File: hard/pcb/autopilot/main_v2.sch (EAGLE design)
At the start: 168 parts, among them IC1 24AA32ASN, IC2 INA194, IC3 LP2950Z, Q1 IRLML5203, Q3 IRLML5203, Q4 IRLML5203, T3 BC848, U2 TMP75DGK, U44 BMP085, X1 USB-SMD-NS

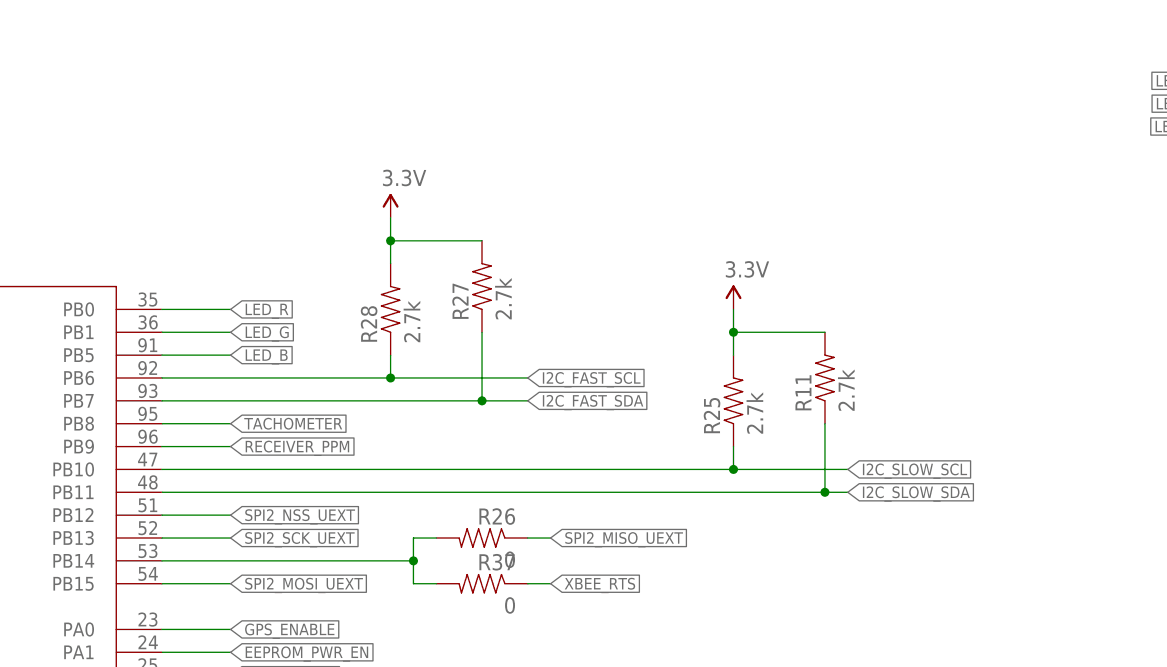
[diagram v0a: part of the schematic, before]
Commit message: nop
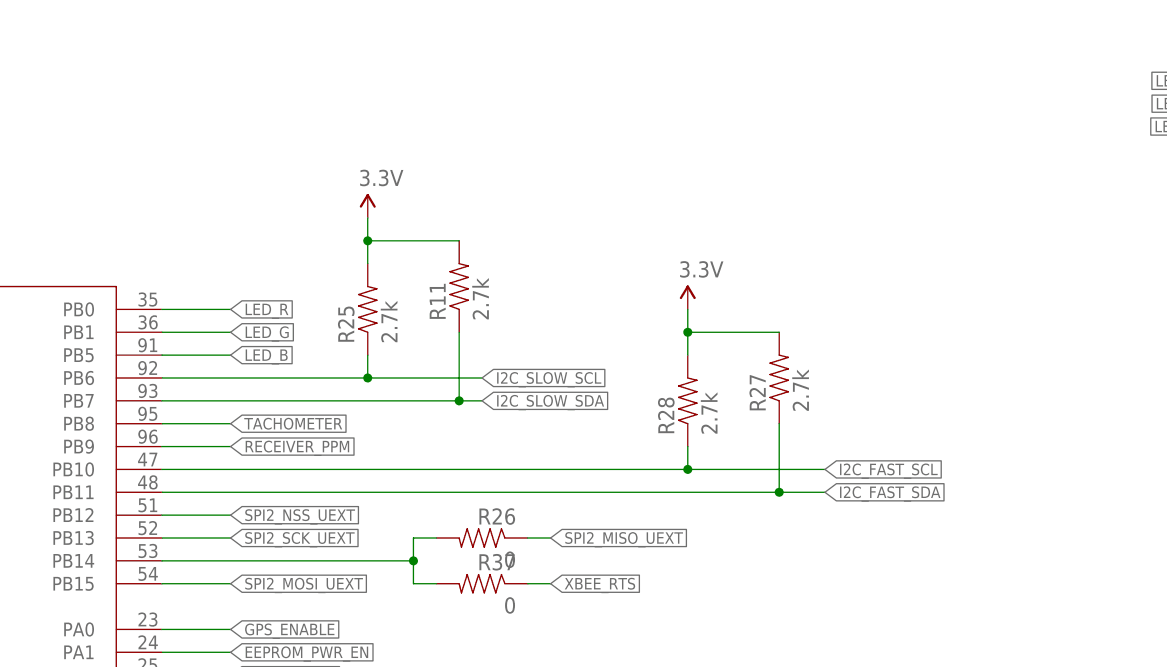
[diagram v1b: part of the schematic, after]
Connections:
- net I2C_FAST_SCL: now also DD1.PB10; no longer DD1.PB6
- net I2C_FAST_SDA: now also DD1.PB11; no longer DD1.PB7
- net I2C_SLOW_SCL: now also DD1.PB6; no longer DD1.PB10
- net I2C_SLOW_SDA: now also DD1.PB7; no longer DD1.PB11
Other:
- moved on the sheet: R11, R25, R27, R28
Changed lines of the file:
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@@
 <setting verticaltext="up"/>
 </settings>
-<grid distance="0.1" unitdist="inch" unit="inch" style="lines" multiple="1" display="no" altdistance="0.01" altunitdist="inch" altunit="inch"/>
+<grid distance="0.1" unitdist="inch" unit="inch" style="lines" multiple="1" display="yes" altdistance="0.01" altunitdist="inch" altunit="inch"/>
 <layers>
 <layer number="1" name="Top" color="4" fill="1" visible="no" active="no"/>
@@
 <instance part="P+18" gate="G$1" x="-218.44" y="2.54"/>
 <instance part="GND31" gate="1" x="-218.44" y="-20.32"/>
-<instance part="R27" gate="G$1" x="76.2" y="78.74" rot="R90"/>
-<instance part="P+16" gate="G$1" x="66.04" y="86.36"/>
-<instance part="R28" gate="G$1" x="66.04" y="76.2" rot="R90"/>
+<instance part="R27" gate="G$1" x="109.22" y="68.58" rot="R90"/>
+<instance part="P+16" gate="G$1" x="99.06" y="76.2"/>
+<instance part="R28" gate="G$1" x="99.06" y="66.04" rot="R90"/>
 <instance part="U44" gate="G$1" x="309.88" y="17.78"/>
 <instance part="U2" gate="G$1" x="309.88" y="-12.7"/>
@@
 <instance part="C37" gate="G$1" x="106.68" y="-55.88" rot="MR180"/>
 <instance part="C39" gate="G$1" x="86.36" y="-55.88" rot="MR180"/>
-<instance part="R11" gate="G$1" x="114.3" y="68.58" rot="R90"/>
-<instance part="P+20" gate="G$1" x="104.14" y="76.2"/>
-<instance part="R25" gate="G$1" x="104.14" y="66.04" rot="R90"/>
+<instance part="R11" gate="G$1" x="73.66" y="78.74" rot="R90"/>
+<instance part="P+20" gate="G$1" x="63.5" y="86.36"/>
+<instance part="R25" gate="G$1" x="63.5" y="76.2" rot="R90"/>
 <instance part="R26" gate="G$1" x="76.2" y="50.8" rot="MR0"/>
 <instance part="R37" gate="G$1" x="76.2" y="45.72" rot="MR0"/>
@@
 </segment>
 <segment>
-<wire x1="66.04" y1="86.36" x2="66.04" y2="83.82" width="0.1524" layer="91"/>
-<wire x1="66.04" y1="83.82" x2="66.04" y2="81.28" width="0.1524" layer="91"/>
-<wire x1="66.04" y1="83.82" x2="76.2" y2="83.82" width="0.1524" layer="91"/>
-<junction x="66.04" y="83.82"/>
+<wire x1="99.06" y1="76.2" x2="99.06" y2="73.66" width="0.1524" layer="91"/>
+<wire x1="99.06" y1="73.66" x2="99.06" y2="71.12" width="0.1524" layer="91"/>
+<wire x1="99.06" y1="73.66" x2="109.22" y2="73.66" width="0.1524" layer="91"/>
+<junction x="99.06" y="73.66"/>
 <pinref part="P+16" gate="G$1" pin="3.3V"/>
 <pinref part="R28" gate="G$1" pin="2"/>
@@
 </segment>
 <segment>
-<wire x1="104.14" y1="76.2" x2="104.14" y2="73.66" width="0.1524" layer="91"/>
-<wire x1="104.14" y1="73.66" x2="104.14" y2="71.12" width="0.1524" layer="91"/>
-<wire x1="104.14" y1="73.66" x2="114.3" y2="73.66" width="0.1524" layer="91"/>
-<junction x="104.14" y="73.66"/>
+<wire x1="63.5" y1="86.36" x2="63.5" y2="83.82" width="0.1524" layer="91"/>
+<wire x1="63.5" y1="83.82" x2="63.5" y2="81.28" width="0.1524" layer="91"/>
+<wire x1="63.5" y1="83.82" x2="73.66" y2="83.82" width="0.1524" layer="91"/>
+<junction x="63.5" y="83.82"/>
 <pinref part="P+20" gate="G$1" pin="3.3V"/>
 <pinref part="R25" gate="G$1" pin="2"/>
@@
 <net name="I2C_FAST_SCL" class="0">
 <segment>
-<wire x1="66.04" y1="71.12" x2="66.04" y2="68.58" width="0.1524" layer="91"/>
-<wire x1="66.04" y1="68.58" x2="81.28" y2="68.58" width="0.1524" layer="91"/>
-<label x="81.28" y="68.58" size="1.27" layer="95" xref="yes"/>
+<wire x1="99.06" y1="60.96" x2="99.06" y2="58.42" width="0.1524" layer="91"/>
+<wire x1="99.06" y1="58.42" x2="114.3" y2="58.42" width="0.1524" layer="91"/>
+<label x="114.3" y="58.42" size="1.27" layer="95" xref="yes"/>
 <pinref part="R28" gate="G$1" pin="1"/>
-<pinref part="DD1" gate="G$1" pin="PB6"/>
-<wire x1="66.04" y1="68.58" x2="40.64" y2="68.58" width="0.1524" layer="91"/>
-<junction x="66.04" y="68.58"/>
+<pinref part="DD1" gate="G$1" pin="PB10"/>
+<wire x1="99.06" y1="58.42" x2="40.64" y2="58.42" width="0.1524" layer="91"/>
+<junction x="99.06" y="58.42"/>
 </segment>
 <segment>
@@
 <net name="I2C_FAST_SDA" class="0">
 <segment>
-<wire x1="76.2" y1="73.66" x2="76.2" y2="66.04" width="0.1524" layer="91"/>
-<wire x1="76.2" y1="66.04" x2="81.28" y2="66.04" width="0.1524" layer="91"/>
-<label x="81.28" y="66.04" size="1.27" layer="95" xref="yes"/>
+<wire x1="109.22" y1="63.5" x2="109.22" y2="55.88" width="0.1524" layer="91"/>
+<wire x1="109.22" y1="55.88" x2="114.3" y2="55.88" width="0.1524" layer="91"/>
+<label x="114.3" y="55.88" size="1.27" layer="95" xref="yes"/>
 <pinref part="R27" gate="G$1" pin="1"/>
-<pinref part="DD1" gate="G$1" pin="PB7"/>
-<wire x1="76.2" y1="66.04" x2="40.64" y2="66.04" width="0.1524" layer="91"/>
-<junction x="76.2" y="66.04"/>
+<pinref part="DD1" gate="G$1" pin="PB11"/>
+<wire x1="109.22" y1="55.88" x2="40.64" y2="55.88" width="0.1524" layer="91"/>
+<junction x="109.22" y="55.88"/>
 </segment>
 <segment>
@@
 <net name="I2C_SLOW_SCL" class="0">
 <segment>
-<label x="116.84" y="58.42" size="1.27" layer="95" xref="yes"/>
+<label x="76.2" y="68.58" size="1.27" layer="95" xref="yes"/>
 <pinref part="R25" gate="G$1" pin="1"/>
-<wire x1="104.14" y1="58.42" x2="116.84" y2="58.42" width="0.1524" layer="91"/>
-<wire x1="104.14" y1="60.96" x2="104.14" y2="58.42" width="0.1524" layer="91"/>
-<junction x="104.14" y="58.42"/>
-<wire x1="104.14" y1="58.42" x2="40.64" y2="58.42" width="0.1524" layer="91"/>
-<pinref part="DD1" gate="G$1" pin="PB10"/>
+<wire x1="63.5" y1="68.58" x2="76.2" y2="68.58" width="0.1524" layer="91"/>
+<wire x1="63.5" y1="71.12" x2="63.5" y2="68.58" width="0.1524" layer="91"/>
+<pinref part="DD1" gate="G$1" pin="PB6"/>
+<wire x1="63.5" y1="68.58" x2="40.64" y2="68.58" width="0.1524" layer="91"/>
+<junction x="63.5" y="68.58"/>
 </segment>
 <segment>
@@
 <net name="I2C_SLOW_SDA" class="0">
 <segment>
-<label x="116.84" y="55.88" size="1.27" layer="95" xref="yes"/>
+<label x="76.2" y="66.04" size="1.27" layer="95" xref="yes"/>
 <pinref part="R11" gate="G$1" pin="1"/>
-<wire x1="114.3" y1="55.88" x2="116.84" y2="55.88" width="0.1524" layer="91"/>
-<wire x1="114.3" y1="63.5" x2="114.3" y2="55.88" width="0.1524" layer="91"/>
-<junction x="114.3" y="55.88"/>
-<wire x1="114.3" y1="55.88" x2="40.64" y2="55.88" width="0.1524" layer="91"/>
-<pinref part="DD1" gate="G$1" pin="PB11"/>
-</segment>
-<segment>
+<wire x1="73.66" y1="66.04" x2="76.2" y2="66.04" width="0.1524" layer="91"/>
+<wire x1="73.66" y1="73.66" x2="73.66" y2="66.04" width="0.1524" layer="91"/>
+<pinref part="DD1" gate="G$1" pin="PB7"/>
+<wire x1="73.66" y1="66.04" x2="40.64" y2="66.04" width="0.1524" layer="91"/>
+<junction x="73.66" y="66.04"/>
+</segment>
+<segment>
